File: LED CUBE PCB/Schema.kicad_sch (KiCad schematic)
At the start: 1 part

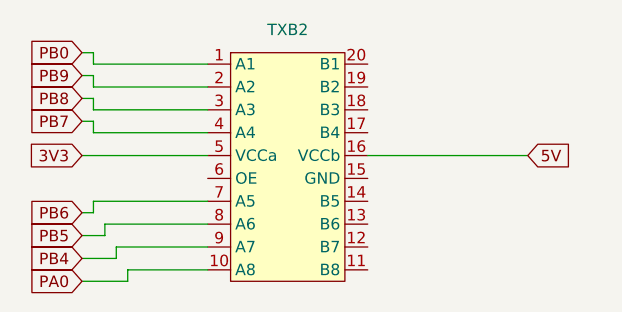
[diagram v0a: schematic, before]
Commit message: Push changes
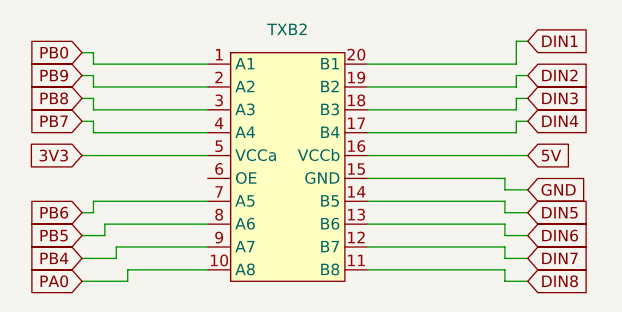
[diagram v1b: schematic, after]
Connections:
- net DIN8: now reaches TXB2.11 (B8)
- net DIN7: now reaches TXB2.12 (B7)
- net DIN6: now reaches TXB2.13 (B6)
- net DIN5: now reaches TXB2.14 (B5)
- net GND: now reaches TXB2.15 (GND)
- net DIN4: now reaches TXB2.17 (B4)
- net DIN3: now reaches TXB2.18 (B3)
- net DIN2: now reaches TXB2.19 (B2)
- net DIN1: now reaches TXB2.20 (B1)
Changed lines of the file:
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@@
 (kicad_sch (version 20230121) (generator eeschema)
   (paper "A4")
+  (wire (pts (xy 153.67 63.5) (xy 156.21 63.5))
+    (stroke (width 0) (type default))
+  )
+  (wire (pts (xy 153.67 52.07) (xy 153.67 53.34))
+    (stroke (width 0) (type default))
+  )
   (wire (pts (xy 120.65 57.15) (xy 109.22 57.15))
     (stroke (width 0) (type default))
   )
+  (wire (pts (xy 154.94 41.91) (xy 154.94 40.64))
+    (stroke (width 0) (type default))
+  )
+  (wire (pts (xy 153.67 58.42) (xy 156.21 58.42))
+    (stroke (width 0) (type default))
+  )
+  (wire (pts (xy 138.43 39.37) (xy 154.94 39.37))
+    (stroke (width 0) (type default))
+  )
   (wire (pts (xy 120.65 39.37) (xy 107.95 39.37))
     (stroke (width 0) (type default))
@@
     (stroke (width 0) (type default))
   )
+  (wire (pts (xy 154.94 43.18) (xy 156.21 43.18))
+    (stroke (width 0) (type default))
+  )
+  (wire (pts (xy 153.67 54.61) (xy 153.67 55.88))
+    (stroke (width 0) (type default))
+  )
   (wire (pts (xy 120.65 59.69) (xy 110.49 59.69))
     (stroke (width 0) (type default))
   )
+  (wire (pts (xy 153.67 53.34) (xy 156.21 53.34))
+    (stroke (width 0) (type default))
+  )
+  (wire (pts (xy 153.67 62.23) (xy 153.67 63.5))
+    (stroke (width 0) (type default))
+  )
   (wire (pts (xy 106.68 43.18) (xy 107.95 43.18))
     (stroke (width 0) (type default))
   )
+  (wire (pts (xy 153.67 59.69) (xy 153.67 60.96))
+    (stroke (width 0) (type default))
+  )
+  (wire (pts (xy 138.43 59.69) (xy 153.67 59.69))
+    (stroke (width 0) (type default))
+  )
   (wire (pts (xy 106.68 63.5) (xy 111.76 63.5))
     (stroke (width 0) (type default))
   )
+  (wire (pts (xy 154.94 39.37) (xy 154.94 36.83))
+    (stroke (width 0) (type default))
+  )
   (wire (pts (xy 120.65 54.61) (xy 107.95 54.61))
     (stroke (width 0) (type default))
   )
+  (wire (pts (xy 138.43 52.07) (xy 153.67 52.07))
+    (stroke (width 0) (type default))
+  )
   (wire (pts (xy 106.68 58.42) (xy 109.22 58.42))
     (stroke (width 0) (type default))
@@
     (stroke (width 0) (type default))
   )
+  (wire (pts (xy 154.94 40.64) (xy 156.21 40.64))
+    (stroke (width 0) (type default))
+  )
+  (wire (pts (xy 138.43 46.99) (xy 154.94 46.99))
+    (stroke (width 0) (type default))
+  )
   (wire (pts (xy 106.68 55.88) (xy 107.95 55.88))
     (stroke (width 0) (type default))
@@
     (stroke (width 0) (type default))
   )
+  (wire (pts (xy 153.67 60.96) (xy 156.21 60.96))
+    (stroke (width 0) (type default))
+  )
   (wire (pts (xy 107.95 41.91) (xy 107.95 40.64))
     (stroke (width 0) (type default))
   )
+  (wire (pts (xy 154.94 45.72) (xy 156.21 45.72))
+    (stroke (width 0) (type default))
+  )
   (wire (pts (xy 106.68 60.96) (xy 110.49 60.96))
     (stroke (width 0) (type default))
   )
+  (wire (pts (xy 154.94 46.99) (xy 154.94 45.72))
+    (stroke (width 0) (type default))
+  )
   (wire (pts (xy 120.65 44.45) (xy 107.95 44.45))
     (stroke (width 0) (type default))
@@
     (stroke (width 0) (type default))
   )
+  (wire (pts (xy 138.43 54.61) (xy 153.67 54.61))
+    (stroke (width 0) (type default))
+  )
   (wire (pts (xy 120.65 62.23) (xy 111.76 62.23))
     (stroke (width 0) (type default))
   )
+  (wire (pts (xy 154.94 44.45) (xy 154.94 43.18))
+    (stroke (width 0) (type default))
+  )
+  (wire (pts (xy 138.43 57.15) (xy 153.67 57.15))
+    (stroke (width 0) (type default))
+  )
   (wire (pts (xy 107.95 39.37) (xy 107.95 38.1))
     (stroke (width 0) (type default))
@@
     (stroke (width 0) (type default))
   )
+  (wire (pts (xy 153.67 55.88) (xy 156.21 55.88))
+    (stroke (width 0) (type default))
+  )
   (wire (pts (xy 107.95 54.61) (xy 107.95 55.88))
     (stroke (width 0) (type default))
@@
     (stroke (width 0) (type default))
   )
+  (wire (pts (xy 154.94 36.83) (xy 156.21 36.83))
+    (stroke (width 0) (type default))
+  )
+  (wire (pts (xy 153.67 57.15) (xy 153.67 58.42))
+    (stroke (width 0) (type default))
+  )
   (wire (pts (xy 111.76 62.23) (xy 111.76 63.5))
     (stroke (width 0) (type default))
   )
+  (wire (pts (xy 138.43 44.45) (xy 154.94 44.45))
+    (stroke (width 0) (type default))
+  )
+  (wire (pts (xy 138.43 41.91) (xy 154.94 41.91))
+    (stroke (width 0) (type default))
+  )
   (wire (pts (xy 107.95 44.45) (xy 107.95 43.18))
     (stroke (width 0) (type default))
@@
     (stroke (width 0) (type default))
   )
+  (wire (pts (xy 138.43 62.23) (xy 153.67 62.23))
+    (stroke (width 0) (type default))
+  )
+  (global_label "GND" (shape input) (at 156.21 53.34 0) (fields_autoplaced)
+    (effects (font (size 1.27 1.27)) (justify left))
+    (property "Intersheetrefs" "${INTERSHEET_REFS}" (at 163.0657 53.34 0)
+      (effects (font (size 1.27 1.27)) (justify left) hide)
+    )
+  )
   (global_label "PB5" (shape input) (at 106.68 58.42 180) (fields_autoplaced)
     (effects (font (size 1.27 1.27)) (justify right))
@@
     )
   )
+  (global_label "DIN4" (shape input) (at 156.21 45.72 0) (fields_autoplaced)
+    (effects (font (size 1.27 1.27)) (justify left))
+    (property "Intersheetrefs" "${INTERSHEET_REFS}" (at 163.61 45.72 0)
+      (effects (font (size 1.27 1.27)) (justify left) hide)
+    )
+  )
   (global_label "PB8" (shape input) (at 106.68 43.18 180) (fields_autoplaced)
     (effects (font (size 1.27 1.27)) (justify right))
@@
     )
   )
+  (global_label "DIN6" (shape input) (at 156.21 58.42 0) (fields_autoplaced)
+    (effects (font (size 1.27 1.27)) (justify left))
+    (property "Intersheetrefs" "${INTERSHEET_REFS}" (at 163.61 58.42 0)
+      (effects (font (size 1.27 1.27)) (justify left) hide)
+    )
+  )
+  (global_label "DIN1" (shape input) (at 156.21 36.83 0) (fields_autoplaced)
+    (effects (font (size 1.27 1.27)) (justify left))
+    (property "Intersheetrefs" "${INTERSHEET_REFS}" (at 163.61 36.83 0)
+      (effects (font (size 1.27 1.27)) (justify left) hide)
+    )
+  )
+  (global_label "DIN7" (shape input) (at 156.21 60.96 0) (fields_autoplaced)
+    (effects (font (size 1.27 1.27)) (justify left))
+    (property "Intersheetrefs" "${INTERSHEET_REFS}" (at 163.61 60.96 0)
+      (effects (font (size 1.27 1.27)) (justify left) hide)
+    )
+  )
   (global_label "PB7" (shape input) (at 106.68 45.72 180) (fields_autoplaced)
     (effects (font (size 1.27 1.27)) (justify right))
@@
     )
   )
+  (global_label "DIN5" (shape input) (at 156.21 55.88 0) (fields_autoplaced)
+    (effects (font (size 1.27 1.27)) (justify left))
+    (property "Intersheetrefs" "${INTERSHEET_REFS}" (at 163.61 55.88 0)
+      (effects (font (size 1.27 1.27)) (justify left) hide)
+    )
+  )
+  (global_label "DIN8" (shape input) (at 156.21 63.5 0) (fields_autoplaced)
+    (effects (font (size 1.27 1.27)) (justify left))
+    (property "Intersheetrefs" "${INTERSHEET_REFS}" (at 163.61 63.5 0)
+      (effects (font (size 1.27 1.27)) (justify left) hide)
+    )
+  )
+  (global_label "DIN2" (shape input) (at 156.21 40.64 0) (fields_autoplaced)
+    (effects (font (size 1.27 1.27)) (justify left))
+    (property "Intersheetrefs" "${INTERSHEET_REFS}" (at 163.61 40.64 0)
+      (effects (font (size 1.27 1.27)) (justify left) hide)
+    )
+  )
   (global_label "PB9" (shape input) (at 106.68 40.64 180) (fields_autoplaced)
     (effects (font (size 1.27 1.27)) (justify right))
@@
     )
   )
+  (global_label "DIN3" (shape input) (at 156.21 43.18 0) (fields_autoplaced)
+    (effects (font (size 1.27 1.27)) (justify left))
+    (property "Intersheetrefs" "${INTERSHEET_REFS}" (at 163.61 43.18 0)
+      (effects (font (size 1.27 1.27)) (justify left) hide)
+    )
+  )
